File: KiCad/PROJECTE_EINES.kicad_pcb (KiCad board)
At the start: 2 copper layers, 107 x 101.9 mm, 63 parts, among them J1 DE9_Pins_MountingHoles, J2 DE9_Pins_MountingHoles, J3 Conn_01x08_Pin, SW1 SS-1GL2-F-D, SW2 SW_DPDT_x2, SW3 SW_DPDT_x2, SW4 SW_DPDT_x2, U1 PIC24HJ128GP504-I_PT, U2 SN65HVD230, U3 VNH5019A-E, U4 LM2596S-5, U5 VNH5019A-E, U6 LM1117DT-3.3, Y1 8MHz

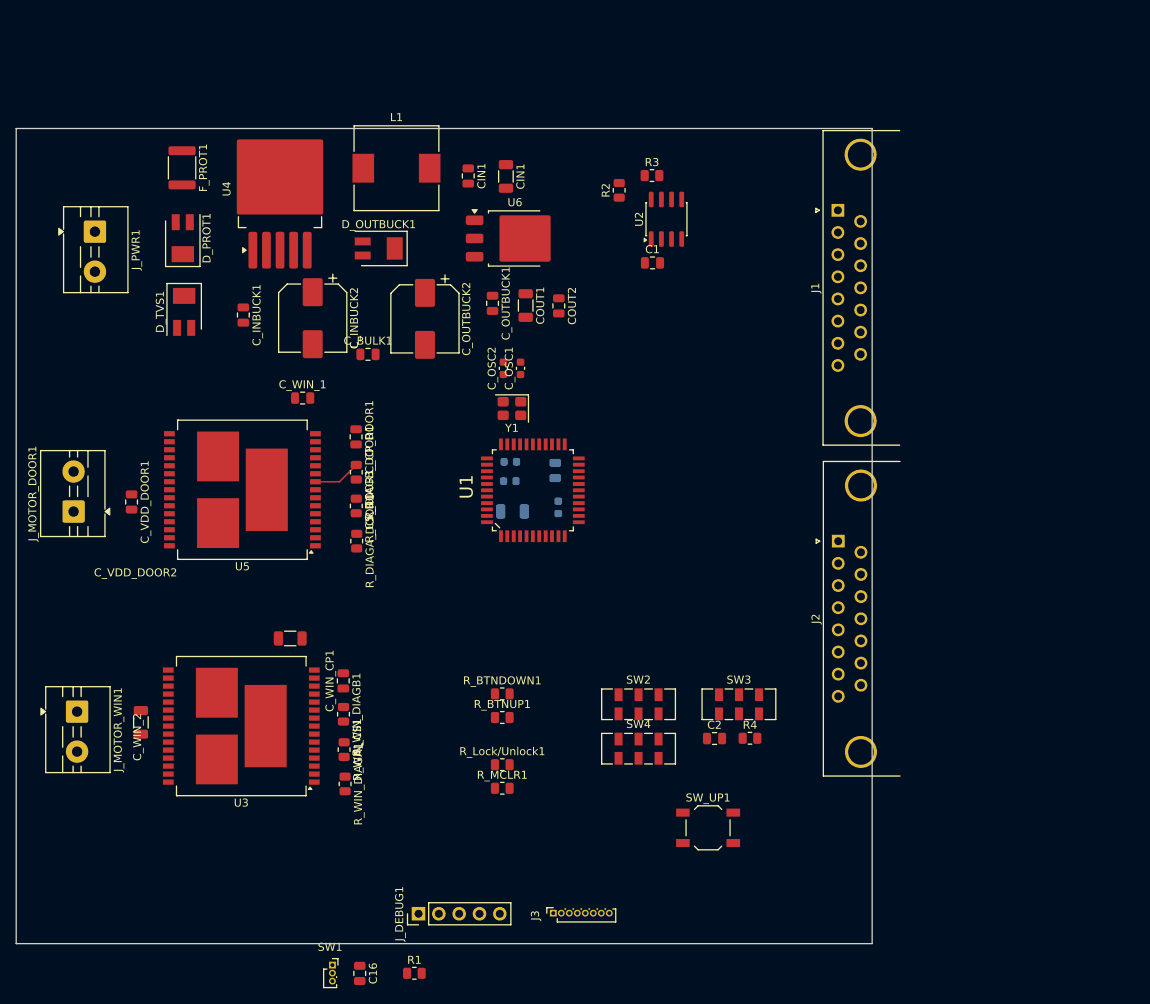
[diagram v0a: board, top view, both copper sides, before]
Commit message: V1 Routing
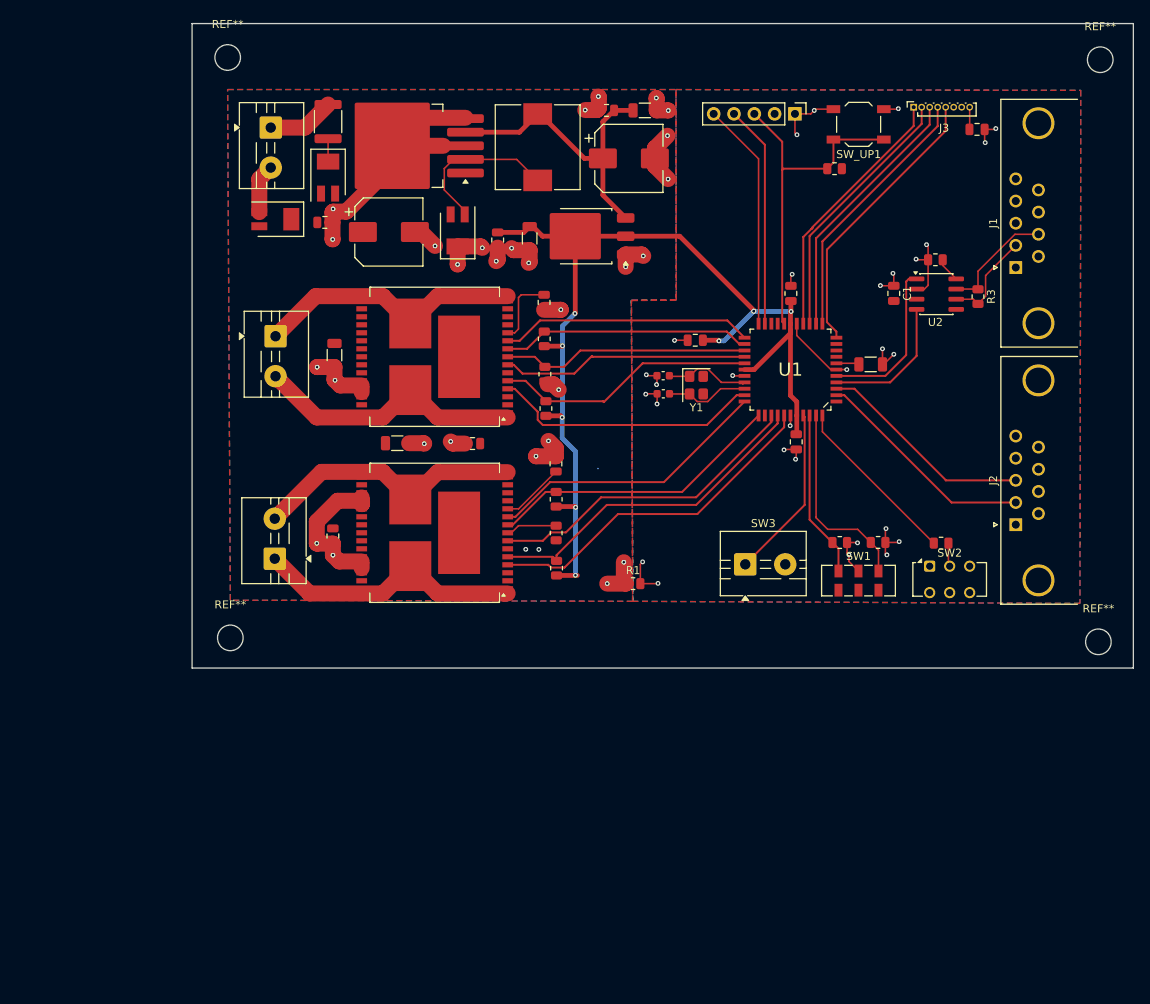
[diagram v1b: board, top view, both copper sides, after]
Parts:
- removed C16: 100n, Capacitor_SMD:C_0805_2012Metric
- removed C2: 100nF, Capacitor_SMD:C_0805_2012Metric
- removed the CIN1 at (118.3, 42.5)
- removed C_VDD2: 100nF, Capacitor_SMD:C_0603_1608Metric
- removed R4: 10k, Resistor_SMD:R_0805_2012Metric
- removed SW4: SW_DPDT_x2, Button_Switch_SMD:SW_DPDT_CK_JS202011JCQN
- added REF**: MountingHole_3.2mm_M3, MountingHole:MountingHole_3.2mm_M3, F.Cu at (88.5, 100.2)
- added REF**: MountingHole_3.2mm_M3, MountingHole:MountingHole_3.2mm_M3, F.Cu at (197.0, 100.7)
- added REF**: MountingHole_3.2mm_M3, MountingHole:MountingHole_3.2mm_M3, F.Cu at (197.3, 27.9)
- added REF**: MountingHole_3.2mm_M3, MountingHole:MountingHole_3.2mm_M3, F.Cu at (88.2, 27.7)
- C3, C_VCAP1: moved to F.Cu
- C_AVDD1, C_VDD1: footprint Capacitor_SMD:C_0603_1608Metric -> Capacitor_SMD:C_0805_2012Metric; moved to F.Cu
- J1, J2: footprint Connector_Dsub:DSUB-15_Socket_Horizontal_P2.77x2.84mm_EdgePinOffset4.94mm_Housed_MountingHolesOffset4.94mm -> Connector_Dsub:DSUB-9_Pins_Horizontal_P2.77x2.84mm_EdgePinOffset4.94mm_Housed_MountingHolesOffset4.94mm
- SW1: value SS-1GL2-F-D -> SW_DPDT_x2; footprint Connector_PinSocket_1.00mm:PinSocket_1x03_P1.00mm_Vertical -> Button_Switch_SMD:SW_DPDT_CK_JS202011JCQN
- SW2: footprint Button_Switch_SMD:SW_DPDT_CK_JS202011JCQN -> Button_Switch_THT:SW_CK_JS202011CQN_DPDT_Straight
- SW3: footprint Button_Switch_SMD:SW_DPDT_CK_JS202011JCQN -> TerminalBlock:TerminalBlock_MaiXu_MX126-5.0-02P_1x02_P5.00mm
- moved J_DEBUG1 110.5 mm to (159.1, 34.7), turned to -90 degrees
- moved J3 110.4 mm to (173.9, 33.9)
- moved SW_UP1 89.9 mm to (167.1, 36.0), turned to 180 degrees
- moved R_MCLR1 87.9 mm to (164.1, 41.6), turned to 180 degrees
- moved SW1 81.4 mm to (167.0, 93.0)
- moved C3 67.8 mm to (181.9, 36.6), turned to 0 degrees
- moved R_Lock/Unlock1 61.4 mm to (177.4, 88.4)
- moved R1 55.9 mm to (138.9, 93.4)
- moved C_BULK1 54.6 mm to (159.3, 75.7), turned to -90 degrees
- moved C_WIN_CP1 53.6 mm to (127.7, 58.3)
- moved R_WIN_CS1 53.2 mm to (127.8, 67.2)
- moved R_WIN_DIAGA1 53.2 mm to (128.0, 71.5)
- moved R_WIN_DIAGB1 53.2 mm to (127.8, 62.8)
- moved J_MOTOR_WIN1 53.1 mm to (94.2, 62.5)
- moved U3 52.1 mm to (114.1, 65.1)
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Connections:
- J3 pad 1: RFID_CS -> RFID_MOSI
- J3 pad 2: RFID_SCK -> RFID_MISO
- J3 pad 3: RFID_MOSI -> RFID_CS
- J3 pad 4: RFID_MISO -> RFID_RST
- J3 pad 5: RFID_RST -> RFID_SCK
- J_DEBUG1 pad 1: MCLR -> GND
- J_DEBUG1 pad 3: GND -> MCLR
- R_Lock/Unlock1 pad 2: Net-(SW4A-B) -> Net-(SW2A-B)
- SW1 pad 1: GND -> WIN_BTN_UP
- SW1 pad 2: unconnected-(SW1-NC-Pad2) -> GND
- SW1 pad 3: WIN_CURRENT_ADC -> WIN_BTN_DOWN
- SW2 pad 1: WIN_BTN_UP -> +3.3V
- SW2 pad 2: GND -> Net-(SW2A-B)
- SW2 pad 3: WIN_BTN_DOWN -> GND
- U1 pad 1: WIN_LIMIT -> unconnected-(U1-SDA1/RP9(1)/CN21/PMD3/RB9-Pad1)
- U1 pad 10: WIN_INB -> unconnected-(U1-AN12/RP12(1)/CN14/PMD0/RB12-Pad10)
- U1 pad 11: WIN_CURRENT_ADC -> RFID_SCK
- U1 pad 12: DOOR_LOCK/UNLOCK -> RFID_RST
- U1 pad 13: unconnected-(U1-TCK/PMA7/RA7-Pad13) -> RFID_CS
- U1 pad 14: WIN_DIAGA -> RFID_MISO
- U1 pad 15: WIN_DIAGB -> RFID_MOSI
- U1 pad 19: RFID_CS -> unconnected-(U1-AN0/VREF+/CN2/RA0-Pad19)
- U1 pad 2: DOOR_DIAGA -> UART_RX
- U1 pad 23: UART_TX -> WIN_INB
- U1 pad 24: UART_RX -> WIN_DIAGB
- U1 pad 25: DOOR_PWM -> WIN_CURRENT_ADC
- U1 pad 26: DOOR_INA -> WIN_PWM
- U1 pad 27: DOOR_INB -> WIN_DIAGA
- U1 pad 3: DOOR_DIAGB -> UART_TX
- U1 pad 32: unconnected-(U1-TDO/PMA8/RA8-Pad32) -> WIN_INA
- U1 pad 33: RFID_MISO -> DOOR_INB
- U1 pad 34: RFID_RST -> DOOR_DIAGB
- U1 pad 36: unconnected-(U1-RP19(1)/CN28/PMBE/RC3-Pad36) -> DOOR_PWM
- U1 pad 37: CAN_RX -> DOOR_DIAGA
- U1 pad 38: CAN_TX -> DOOR_INA
- U1 pad 4: unconnected-(U1-RP24(1)/CN20/PMA5/RC8-Pad4) -> CAN_RX
- U1 pad 41: RFID_MOSI -> WIN_LIMIT
- U1 pad 42: RFID_SCK -> WIN_BTN_UP
- U1 pad 43: WIN_BTN_UP -> WIN_BTN_DOWN
- U1 pad 44: WIN_BTN_DOWN -> DOOR_LOCK/UNLOCK
- U1 pad 5: unconnected-(U1-RP25(1)/CN19/PMA6/RC9-Pad5) -> CAN_TX
- U1 pad 8: WIN_PWM -> unconnected-(U1-PGED2/EMCD2/RP10(1)/CN16/PMD2/RB10-Pad8)
- U1 pad 9: WIN_INA -> unconnected-(U1-PGEC2/RP11(1)/CN15/PMD1/RB11-Pad9)
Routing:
- net +3.3V: track 0.00 -> 131.2 mm, vias 0 -> 9
- net GNDPWR: track 0.00 -> 114.1 mm, vias 0 -> 30
- net GND: track 0.00 -> 67.5 mm, vias 0 -> 29
- net MCLR: track 0.00 -> 43.7 mm
- net DOOR_INA: track 0.00 -> 43.4 mm
- net DOOR_DIAGA: track 0.00 -> 42.5 mm
- net DOOR_PWM: track 0.00 -> 39.9 mm
- net +5V: track 0.00 -> 38.0 mm
- net DOOR_INB: track 0.00 -> 35.6 mm
- net RFID_SCK: track 0.00 -> 35.5 mm
- net DOOR_MOTOR_B: track 0.00 -> 34.4 mm
- net WIN_MOTOR_B: track 0.00 -> 34.0 mm
- net WIN_MOTOR_A: track 0.00 -> 33.9 mm
- net DOOR_MOTOR_A: track 0.00 -> 33.7 mm
- net WIN_INA: track 0.00 -> 33.6 mm
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- added copper zone on F.Cu, net +3.3V
- added copper zone on B.Cu, net GND
- added copper zone on B.Cu, net GNDPWR
- added copper zone on F.Cu, net VBAT_PROT
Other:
- board size 107 x 101.9 mm -> 117.7 x 80.6 mm

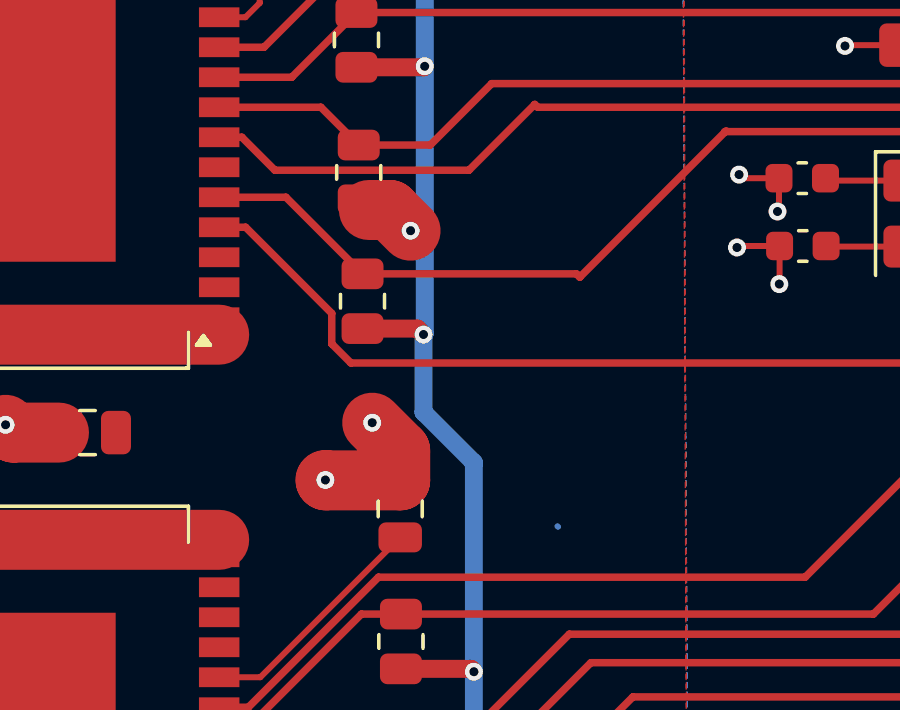
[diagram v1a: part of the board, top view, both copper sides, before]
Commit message: V2 Routing
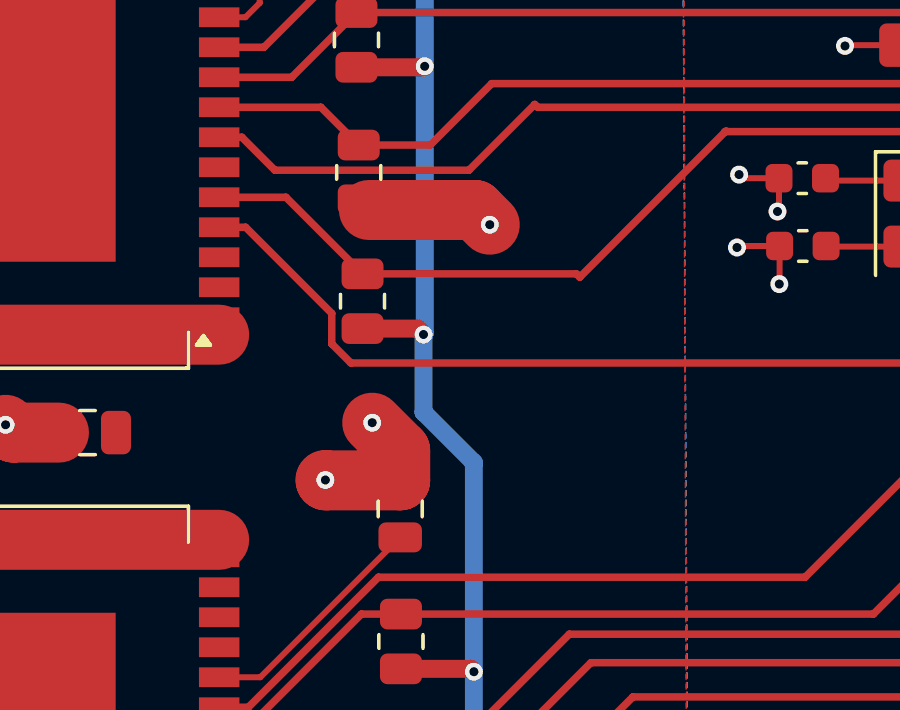
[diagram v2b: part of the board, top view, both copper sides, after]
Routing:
- net GNDPWR: track 114.1 -> 116.7 mm
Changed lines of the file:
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@@
+	)
+	(segment
+		(start 131.7201 68.5001)
+		(end 128.1808 68.5001)
+		(width 2)
+		(layer "F.Cu")
+		(net 3)
 	)
 	(segment
@@
 	)
 	(segment
-		(start 129.57 69.19)
-		(end 128.8801 68.5001)
-		(width 2)
-		(layer "F.Cu")
-		(net 3)
-	)
-	(segment
 		(start 104.94 83.075)
 		(end 104.94 82.656)
@@
 	)
 	(segment
+		(start 132.21 68.99)
+		(end 131.7201 68.5001)
+		(width 2)
+		(layer "F.Cu")
+		(net 3)
+	)
+	(segment
 		(start 125.94 51.75)
 		(end 123.94 51.75)
@@
 	)
 	(segment
-		(start 128.8801 68.5001)
-		(end 128.1808 68.5001)
-		(width 2)
-		(layer "F.Cu")
-		(net 3)
-	)
-	(segment
 		(start 125.94 51.75)
 		(end 125.94 53.22)
@@
 	)
 	(via
-		(at 129.57 69.19)
+		(at 132.21 68.99)
 		(size 0.6)
 		(drill 0.3)
@@
 		(net 7)
 	)
-	(segment
-		(start 134.4665 79.04)
-		(end 134.4865 79.06)
-		(width 0.2)
-		(layer "B.Cu")
-		(net 7)
-	)
